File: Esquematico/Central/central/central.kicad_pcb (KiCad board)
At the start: 2 copper layers, 145.2 x 84.8 mm, 69 parts, among them J1 Conn_01x03_Socket, J2 Conn_01x03_Socket, J3 Conn_01x03_Socket, J4 Conn_01x03_Socket, J5 USB_A, K1 JQC-3FF-005-1Z, K2 JQC-3FF-005-1Z, K3 JQC-3FF-005-1Z, Q1 2TY, Q2 2TY, Q3 2TY, U1 ESP32-S3-WROOM-1, U2 AMS1117-3.3

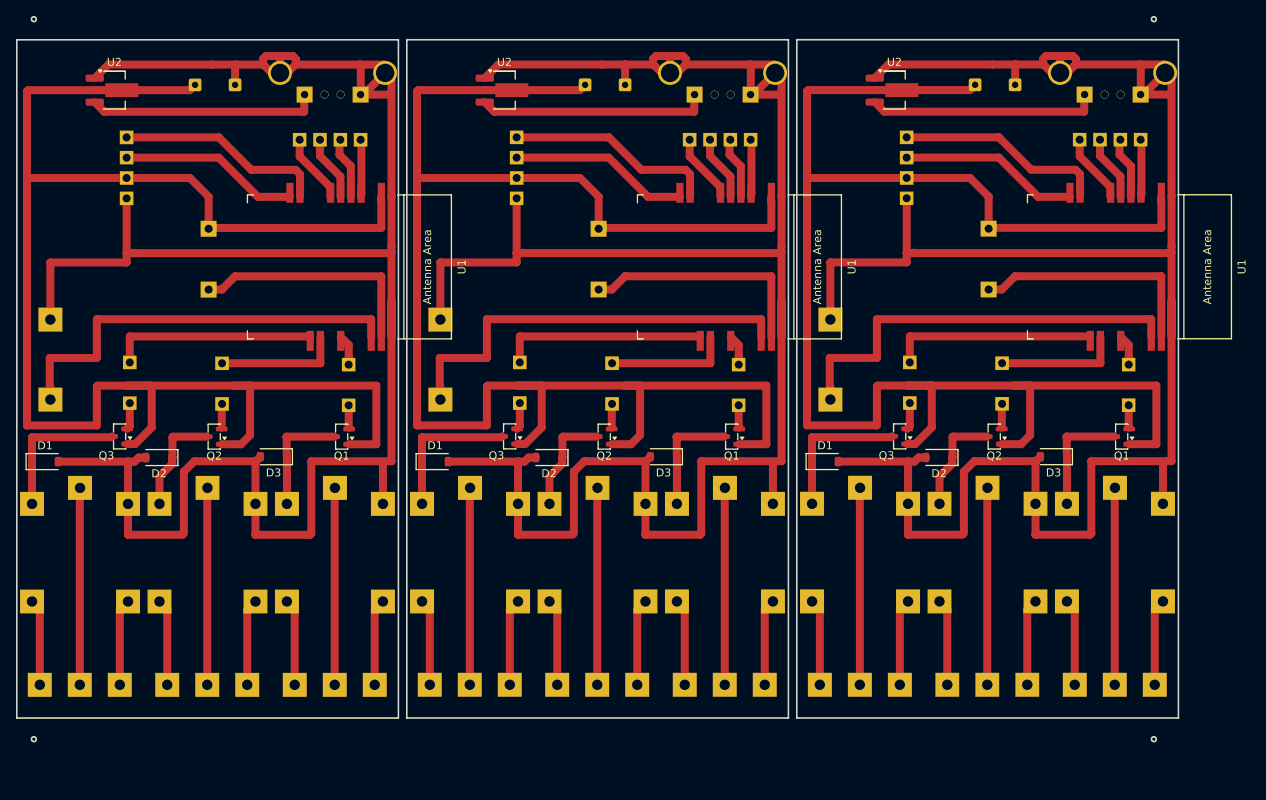
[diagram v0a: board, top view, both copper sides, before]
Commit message: Commit automático
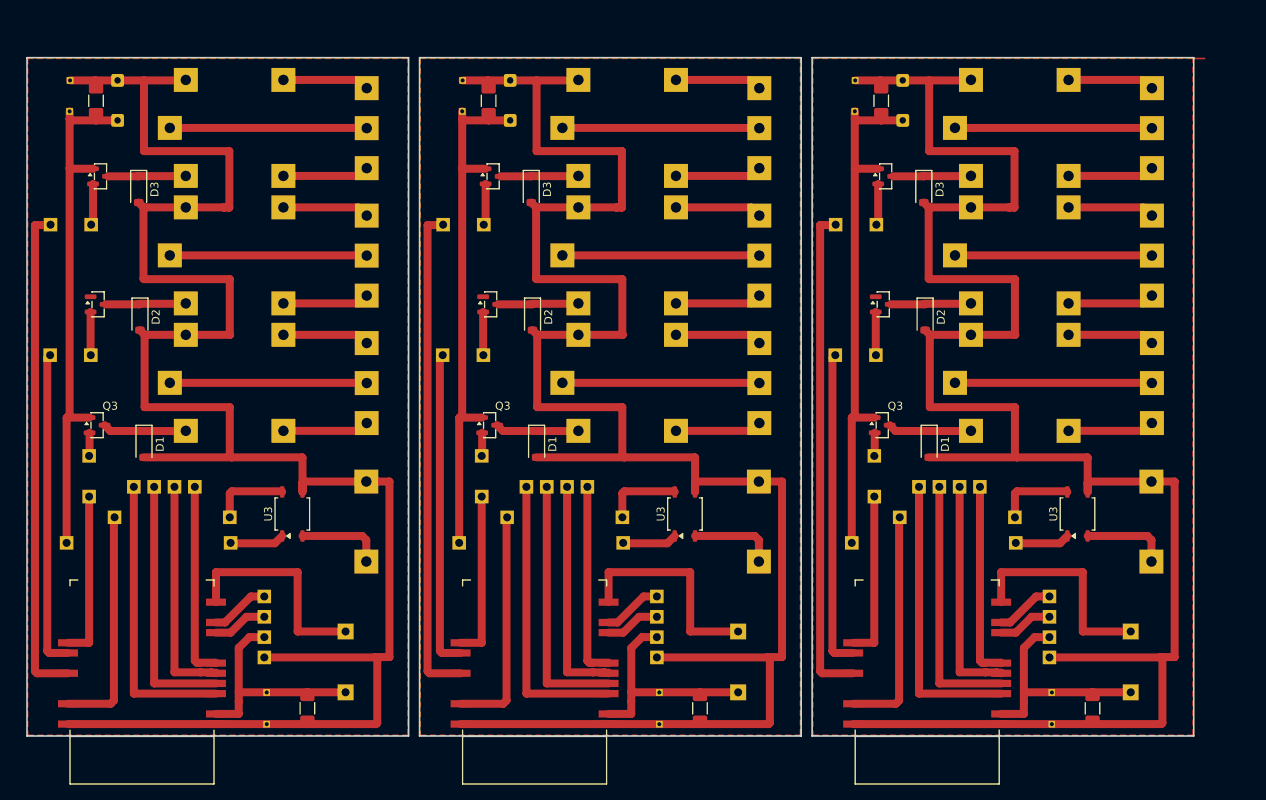
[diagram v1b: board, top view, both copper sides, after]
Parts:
- removed the BZ1 at (136.0, 79.5)
- removed the BZ1 at (184.7, 79.5)
- removed the Brd1 at (115.1, 72.1)
- removed the Brd1 at (163.9, 72.1)
- removed the C1 at (183.0, 61.5)
- removed the C1 at (134.3, 61.5)
- removed the C1 at (85.5, 61.5)
- removed the D1 at (115.5, 108.6)
- removed the D1 at (164.3, 108.6)
- removed the D2 at (178.5, 108.1)
- removed the D2 at (129.8, 108.1)
- removed the D3 at (144.1, 108.0)
- removed the D3 at (192.8, 108.0)
- removed the J1 at (205.5, 136.5)
- removed the J1 at (156.7, 136.5)
- removed the J2 at (140.8, 136.5)
- removed the J2 at (189.6, 136.5)
- removed the J3 at (173.6, 136.5)
- removed the J3 at (124.9, 136.5)
- removed the J4 at (164.9, 100.9)
- removed the J4 at (116.2, 100.9)
- removed the J5 at (148.0, 62.7)
- removed the J5 at (196.7, 62.7)
- removed the J5 at (99.2, 62.7)
- removed the Jtouch1 at (196.1, 68.4)
- removed the Jtouch1 at (147.4, 68.4)
- removed the K1 at (194.5, 113.9)
- removed the K1 at (145.8, 113.9)
- removed the K2 at (178.6, 113.9)
- removed the K2 at (129.8, 113.9)
- removed the K3 at (162.7, 113.9)
- removed the K3 at (113.9, 113.9)
- removed the Q1 at (201.4, 105.5)
- removed the Q1 at (152.6, 105.5)
- removed the Q2 at (136.7, 105.5)
- removed the Q2 at (185.4, 105.5)
- removed the Q3 at (173.6, 105.5)
- removed the Q3 at (124.9, 105.5)
- removed the R1 at (153.5, 96.5)
- removed the R1 at (202.2, 96.5)
- removed the R2 at (137.7, 96.3)
- removed the R2 at (186.4, 96.3)
- removed the R3 at (174.9, 96.2)
- removed the R3 at (126.1, 96.2)
- removed the U1 at (150.6, 84.3)
- removed the U1 at (199.3, 84.3)
- removed U2 (x3): AMS1117-3.3, Package_TO_SOT_SMD:SOT-89-3_Handsoldering
- added BZ1: Buzzer, Buzzer_Beeper:Buzzer_15x7.5RM7.6, B.Cu at (153.4, 137.4)
- added BZ1: Buzzer, Buzzer_Beeper:Buzzer_15x7.5RM7.6, B.Cu at (202.5, 137.4)
- added Brd1: SSD1306, SSD1306:128x64OLED, B.Cu at (181.7, 129.5)
- added Brd1: SSD1306, SSD1306:128x64OLED, B.Cu at (132.7, 129.5)
- added C1: 470u, Capacitor_THT:CP_Radial_D8.0mm_P5.00mm, B.Cu at (174.0, 66.0)
- added C1: 470u, Capacitor_THT:CP_Radial_D8.0mm_P5.00mm, B.Cu at (124.9, 66.0)
- added C1: 470u, Capacitor_THT:CP_Radial_D8.0mm_P5.00mm, B.Cu at (75.8, 66.0)
- added C2: 100n, Capacitor_SMD:C_1206_3216Metric_Pad1.33x1.80mm_HandSolder, F.Cu at (171.3, 63.5)
- added C2: 100n, Capacitor_SMD:C_1206_3216Metric_Pad1.33x1.80mm_HandSolder, F.Cu at (73.2, 63.5)
- added C2: 100n, Capacitor_SMD:C_1206_3216Metric_Pad1.33x1.80mm_HandSolder, F.Cu at (122.2, 63.5)
- added C3: 100n, Capacitor_SMD:C_1206_3216Metric_Pad1.33x1.80mm_HandSolder, F.Cu at (99.6, 139.4)
- added C3: 100n, Capacitor_SMD:C_1206_3216Metric_Pad1.33x1.80mm_HandSolder, F.Cu at (197.7, 139.4)
- added C3: 100n, Capacitor_SMD:C_1206_3216Metric_Pad1.33x1.80mm_HandSolder, F.Cu at (148.6, 139.4)
- added D1: 1N4148, Diode_SMD:D_SOD-123, F.Cu at (177.3, 106.4)
- added D1: 1N4148, Diode_SMD:D_SOD-123, F.Cu at (128.2, 106.4)
- added D2: 1N4148, Diode_SMD:D_SOD-123, F.Cu at (127.7, 90.5)
- added D2: 1N4148, Diode_SMD:D_SOD-123, F.Cu at (176.8, 90.5)
- added D3: 1N4148, Diode_SMD:D_SOD-123, F.Cu at (176.6, 74.6)
- added D3: 1N4148, Diode_SMD:D_SOD-123, F.Cu at (127.6, 74.6)
- added J1: Conn_01x03_Socket, TerminalBlock_MetzConnect:TerminalBlock_MetzConnect_Type094_RT03503HBLU_1x03_P5.00mm_Horizontal, B.Cu at (156.1, 61.9)
- added J1: Conn_01x03_Socket, TerminalBlock_MetzConnect:TerminalBlock_MetzConnect_Type094_RT03503HBLU_1x03_P5.00mm_Horizontal, B.Cu at (205.1, 61.9)
- added J2: Conn_01x03_Socket, TerminalBlock_MetzConnect:TerminalBlock_MetzConnect_Type094_RT03503HBLU_1x03_P5.00mm_Horizontal, B.Cu at (156.1, 77.9)
- added J2: Conn_01x03_Socket, TerminalBlock_MetzConnect:TerminalBlock_MetzConnect_Type094_RT03503HBLU_1x03_P5.00mm_Horizontal, B.Cu at (205.1, 77.9)
- added J3: Conn_01x03_Socket, TerminalBlock_MetzConnect:TerminalBlock_MetzConnect_Type094_RT03503HBLU_1x03_P5.00mm_Horizontal, B.Cu at (156.1, 93.8)
- added J3: Conn_01x03_Socket, TerminalBlock_MetzConnect:TerminalBlock_MetzConnect_Type094_RT03503HBLU_1x03_P5.00mm_Horizontal, B.Cu at (205.1, 93.8)
- added J4: Conn_01x03_Socket, TerminalBlock_MetzConnect:TerminalBlock_MetzConnect_Type094_RT03503HBLU_1x03_P5.00mm_Horizontal, B.Cu at (156.0, 111.1)
- added J4: Conn_01x03_Socket, TerminalBlock_MetzConnect:TerminalBlock_MetzConnect_Type094_RT03503HBLU_1x03_P5.00mm_Horizontal, B.Cu at (205.1, 111.1)
- added J5: Conn_01x01_Pin, Connector_PinHeader_1.00mm:PinHeader_1x01_P1.00mm_Vertical, B.Cu at (69.8, 64.8)
- added J5: Conn_01x01_Pin, Connector_PinHeader_1.00mm:PinHeader_1x01_P1.00mm_Vertical, B.Cu at (118.9, 64.8)
- added J5: Conn_01x01_Pin, Connector_PinHeader_1.00mm:PinHeader_1x01_P1.00mm_Vertical, B.Cu at (168.0, 64.8)
- added J6: Conn_01x01_Pin, Connector_PinHeader_1.00mm:PinHeader_1x01_P1.00mm_Vertical, B.Cu at (69.9, 61.0)
- added J6: Conn_01x01_Pin, Connector_PinHeader_1.00mm:PinHeader_1x01_P1.00mm_Vertical, B.Cu at (168.0, 61.0)
- added J6: Conn_01x01_Pin, Connector_PinHeader_1.00mm:PinHeader_1x01_P1.00mm_Vertical, B.Cu at (119.0, 61.0)
- added J7: Conn_01x01_Pin, Connector_PinHeader_1.00mm:PinHeader_1x01_P1.00mm_Vertical, B.Cu at (143.6, 137.5)
- added J7: Conn_01x01_Pin, Connector_PinHeader_1.00mm:PinHeader_1x01_P1.00mm_Vertical, B.Cu at (94.5, 137.5)
- added J7: Conn_01x01_Pin, Connector_PinHeader_1.00mm:PinHeader_1x01_P1.00mm_Vertical, B.Cu at (192.6, 137.5)
- added J8: Conn_01x01_Pin, Connector_PinHeader_1.00mm:PinHeader_1x01_P1.00mm_Vertical, B.Cu at (94.5, 141.4)
- added J8: Conn_01x01_Pin, Connector_PinHeader_1.00mm:PinHeader_1x01_P1.00mm_Vertical, B.Cu at (192.6, 141.4)
- added J8: Conn_01x01_Pin, Connector_PinHeader_1.00mm:PinHeader_1x01_P1.00mm_Vertical, B.Cu at (143.6, 141.4)
- added Jtouch1: Conn_01x04_Pin, Connector_PinHeader_2.54mm:PinHeader_1x04_P2.54mm_Vertical, B.Cu at (134.6, 111.8)
- added Jtouch1: Conn_01x04_Pin, Connector_PinHeader_2.54mm:PinHeader_1x04_P2.54mm_Vertical, B.Cu at (183.6, 111.8)
- added K1: JQC-3FF-005-1Z, Relay_THT:Relay_SPDT_Hongfa_JQC-3FF_0XX-1Z, B.Cu at (133.4, 72.9)
- added K1: JQC-3FF-005-1Z, Relay_THT:Relay_SPDT_Hongfa_JQC-3FF_0XX-1Z, B.Cu at (182.5, 72.9)
- added K2: JQC-3FF-005-1Z, Relay_THT:Relay_SPDT_Hongfa_JQC-3FF_0XX-1Z, B.Cu at (182.5, 88.8)
- added K2: JQC-3FF-005-1Z, Relay_THT:Relay_SPDT_Hongfa_JQC-3FF_0XX-1Z, B.Cu at (133.4, 88.8)
- added K3: JQC-3FF-005-1Z, Relay_THT:Relay_SPDT_Hongfa_JQC-3FF_0XX-1Z, B.Cu at (133.4, 104.8)
- added K3: JQC-3FF-005-1Z, Relay_THT:Relay_SPDT_Hongfa_JQC-3FF_0XX-1Z, B.Cu at (182.5, 104.8)
- added Q1: 2TY, Package_TO_SOT_SMD:SOT-23, F.Cu at (122.8, 72.9)
- added Q1: 2TY, Package_TO_SOT_SMD:SOT-23, F.Cu at (171.9, 72.9)
- added Q2: 2TY, Package_TO_SOT_SMD:SOT-23, F.Cu at (122.5, 89.0)
- added Q2: 2TY, Package_TO_SOT_SMD:SOT-23, F.Cu at (171.6, 89.0)
- added Q3: 2TY, Package_TO_SOT_SMD:SOT-23, F.Cu at (171.4, 104.1)
- added Q3: 2TY, Package_TO_SOT_SMD:SOT-23, F.Cu at (122.3, 104.1)
- added R1: 2K, Resistor_THT:R_Axial_DIN0204_L3.6mm_D1.6mm_P5.08mm_Horizontal, B.Cu at (116.5, 79.0)
- added R1: 2K, Resistor_THT:R_Axial_DIN0204_L3.6mm_D1.6mm_P5.08mm_Horizontal, B.Cu at (165.6, 79.0)
- added R2: 2K, Resistor_THT:R_Axial_DIN0204_L3.6mm_D1.6mm_P5.08mm_Horizontal, B.Cu at (116.5, 95.3)
- added R2: 2K, Resistor_THT:R_Axial_DIN0204_L3.6mm_D1.6mm_P5.08mm_Horizontal, B.Cu at (165.6, 95.3)
- added R3: 2K, Resistor_THT:R_Axial_DIN0204_L3.6mm_D1.6mm_P5.08mm_Horizontal, B.Cu at (170.4, 113.0)
- added R3: 2K, Resistor_THT:R_Axial_DIN0204_L3.6mm_D1.6mm_P5.08mm_Horizontal, B.Cu at (121.4, 113.0)
- added R4: 470R, Resistor_THT:R_Axial_DIN0309_L9.0mm_D3.2mm_P12.70mm_Horizontal, B.Cu at (118.5, 118.8)
- added R4: 470R, Resistor_THT:R_Axial_DIN0309_L9.0mm_D3.2mm_P12.70mm_Horizontal, B.Cu at (69.5, 118.8)
- added R4: 470R, Resistor_THT:R_Axial_DIN0309_L9.0mm_D3.2mm_P12.70mm_Horizontal, B.Cu at (167.6, 118.8)
- added R5: 100R, Resistor_THT:R_Axial_DIN0309_L9.0mm_D3.2mm_P12.70mm_Horizontal, B.Cu at (89.9, 115.6)
- added R5: 100R, Resistor_THT:R_Axial_DIN0309_L9.0mm_D3.2mm_P12.70mm_Horizontal, B.Cu at (138.9, 115.6)
- added R5: 100R, Resistor_THT:R_Axial_DIN0309_L9.0mm_D3.2mm_P12.70mm_Horizontal, B.Cu at (188.0, 115.6)
- added U1: ESP32-S3-WROOM-1, PCM_Espressif:ESP32-S3-WROOM-1, F.Cu at (128.0, 133.2)
- added U1: ESP32-S3-WROOM-1, PCM_Espressif:ESP32-S3-WROOM-1, F.Cu at (177.0, 133.2)
- added U3: EL817, Package_SO:SOP-4_3.8x4.1mm_P2.54mm, F.Cu at (146.8, 115.2)
- added U3: EL817, Package_SO:SOP-4_3.8x4.1mm_P2.54mm, F.Cu at (97.7, 115.2)
- added U3: EL817, Package_SO:SOP-4_3.8x4.1mm_P2.54mm, F.Cu at (195.8, 115.2)
- R1, R2, R3: value 242 -> 2K
- moved J1 74.6 mm to (107.0, 61.9), turned to -90 degrees
- moved J2 60.5 mm to (107.0, 77.9), turned to -90 degrees
- moved BZ1 60.4 mm to (104.3, 137.4), turned to 90 degrees
- moved Brd1 59.9 mm to (83.6, 129.5)
- moved U1 54.0 mm to (78.9, 133.2), turned to 180 degrees
- moved J3 52.7 mm to (107.0, 93.8), turned to -90 degrees
- moved Jtouch1 45.3 mm to (85.5, 111.8), turned to 90 degrees
- moved Q1 44.4 mm to (73.7, 72.9), turned to 0 degrees
- moved K1 42.9 mm to (84.4, 72.9), turned to 0 degrees
- moved R1 41.2 mm to (67.5, 79.0), turned to 0 degrees
- moved J4 40.8 mm to (106.9, 111.1), turned to -90 degrees
- moved D3 37.4 mm to (78.5, 74.6), turned to -90 degrees
- moved K2 25.3 mm to (84.4, 88.8), turned to 0 degrees
- moved Q2 22.0 mm to (73.4, 89.0), turned to 0 degrees
- moved R2 21.5 mm to (67.4, 95.3), turned to 0 degrees
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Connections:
- J4 pad 1: Net-(J4-Pin_1) -> GND
- J4 pad 3: GND -> Net-(J4-Pin_3)
- Q1 pad 1: VCC -> +5V
- Q2 pad 1: VCC -> +5V
- Q3 pad 1: VCC -> +5V
- U1 pad 10: Net-(Brd1-SDA) -> Net-(Brd1-SCL)
- U1 pad 11: Net-(Brd1-SCL) -> Net-(Brd1-SDA)
- U1 pad 38: Net-(J4-Pin_1) -> Net-(U1-GPIO2/TOUCH2/ADC1_CH1)
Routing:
- net VCC: track 600.4 -> 86.2 mm
- net +5V: track 0.00 -> 200.5 mm
- net Net-(U1-MTMS/GPIO42): track 11.7 -> 185.8 mm
- net Net-(J4-Pin_1): track 157.4 -> 0.00 mm
- net Net-(Jtouch1-Pin_4): track 21.6 -> 108.4 mm
- net Net-(U1-GPIO2/TOUCH2/ADC1_CH1): track 0.00 -> 86.5 mm
- net Net-(J5-VBUS): track 86.4 -> 0.00 mm
- net Net-(Jtouch1-Pin_3): track 23.3 -> 96.9 mm
- net Net-(U1-MTDO/GPIO40/CLK_OUT2): track 46.8 -> 119.5 mm
- net Net-(Jtouch1-Pin_2): track 24.6 -> 85.4 mm
- net GND: track 775.6 -> 717.6 mm
- net Net-(Brd1-SDA): track 79.2 -> 22.1 mm
- net Net-(Jtouch1-Pin_1): track 26.2 -> 73.5 mm
- net Net-(Brd1-SCL): track 67.3 -> 20.6 mm
- net Net-(J4-Pin_3): track 0.00 -> 32.6 mm
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- added copper zone on F.Cu, net GND
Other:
- board size 145.2 x 84.8 mm -> 145.8 x 84.8 mm
